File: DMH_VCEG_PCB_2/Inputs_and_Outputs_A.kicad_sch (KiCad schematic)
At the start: 43 parts, among them J1 TS_Jack_6.35mm_Sw, J10 TS_Jack_6.35mm_Sw, J2 TS_Jack_6.35mm_Sw, J200 IDC_02x08, J21 Conn_01x10_PinHeader, J22 Conn_01x10_PinHeader, J23 Conn_01x10_PinHeader, J24 Conn_01x06_PinHeader, J3 TS_Jack_6.35mm_Sw, J4 TS_Jack_6.35mm_Sw, J5 TS_Jack_6.35mm_Sw, J6 TS_Jack_6.35mm_Sw, J7 TS_Jack_6.35mm_Sw, J8 TS_Jack_6.35mm_Sw, J9 TS_Jack_6.35mm_Sw, U21 TL074, U7 TL074, U8 TL074

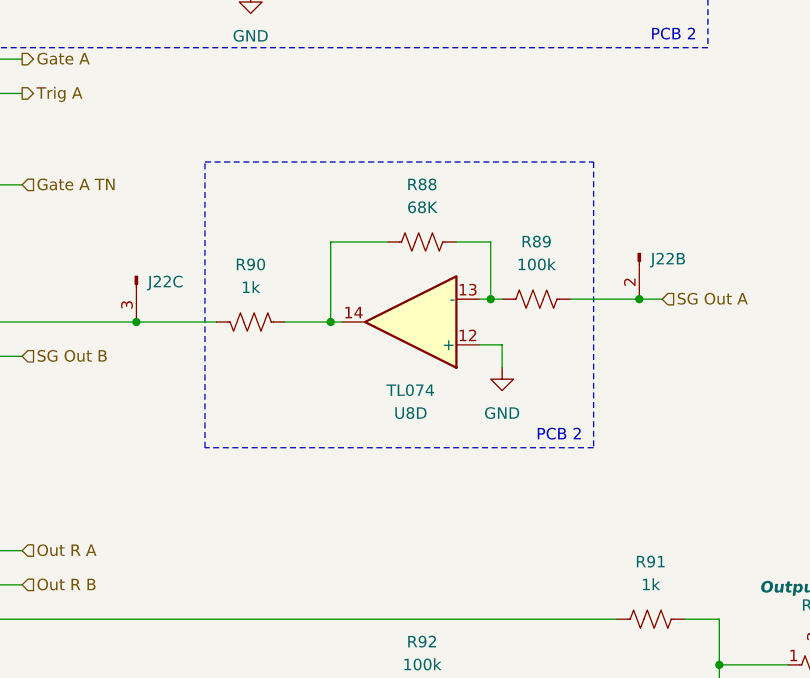
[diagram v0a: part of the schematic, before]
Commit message: Synced changes to PCB 2
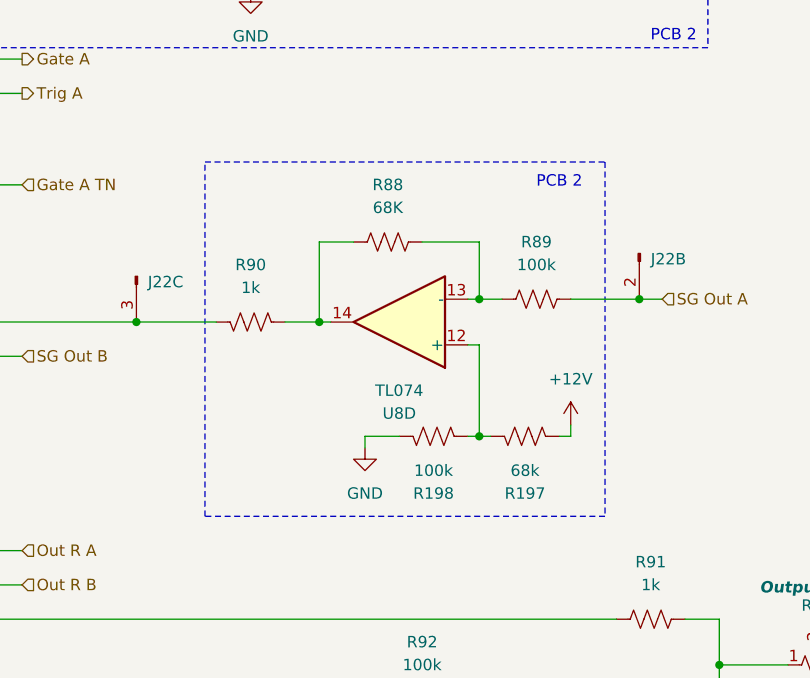
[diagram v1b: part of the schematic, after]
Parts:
- added R197: 68k, Resistor_THT:R_Axial_DIN0207_L6.3mm_D2.5mm_P7.62mm_Horizontal, symbol Device:R_US
- added R198: 100k, Resistor_THT:R_Axial_DIN0207_L6.3mm_D2.5mm_P7.62mm_Horizontal, symbol Device:R_US
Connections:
- net +12V: now also R197.1
- net GND: now also R198.2; no longer U8.12 (+)
- new net: R197.2, R198.1, U8.12 (+)
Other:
- moved on the sheet: R88, U8D
